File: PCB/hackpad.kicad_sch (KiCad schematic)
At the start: 8 parts, among them SW1 SW_Push, SW2 SW_Push, SW3 SW_Push, SW4 SW_Push, SW5 SW_Push, U1 XIAO-RP2040-DIP

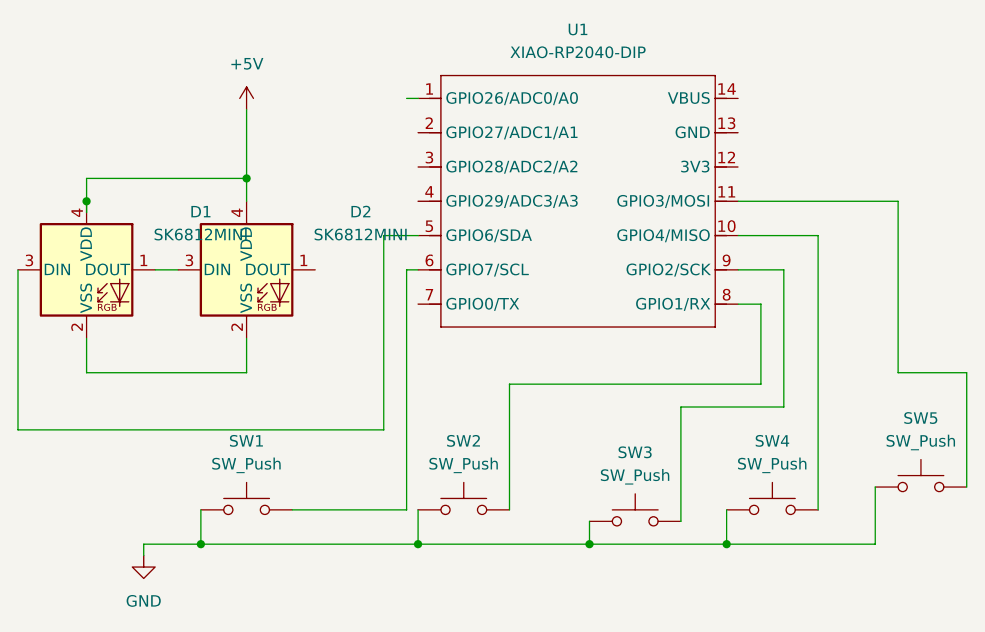
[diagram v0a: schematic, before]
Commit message: Add files via upload
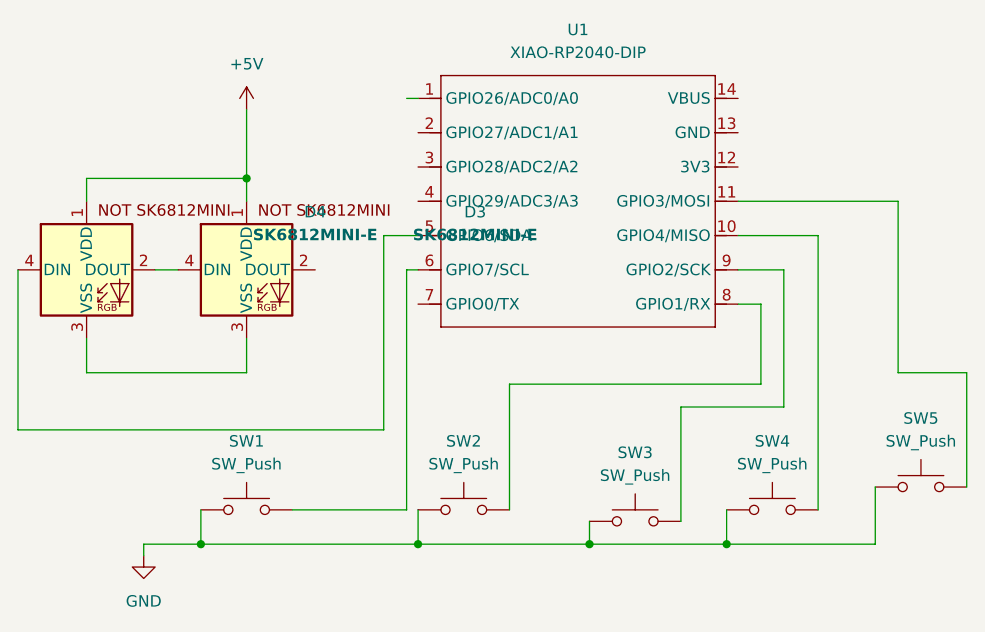
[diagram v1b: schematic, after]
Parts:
- removed D1, D2: SK6812MINI, LED_SMD:LED_SK6812MINI_PLCC4_3.5x3.5mm_P1.75mm, symbol LED:SK6812MINI
- added D3, D4: SK6812MINI-E, SK6812MINI-E - 3.2x2.8x1.78mm, symbol SK6812MINI E:SK6812MINI-E
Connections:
- net +5V: now also D3.1 (VDD), D4.1 (VDD)
- net at U1.5 (GPIO6/SDA): now also D4.4 (DIN)
- new net: D3.3 (VSS), D4.3 (VSS)
- new net: D3.4 (DIN), D4.2 (DOUT)
